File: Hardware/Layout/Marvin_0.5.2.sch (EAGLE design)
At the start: 56 parts, among them IC1 LM321MF, Q1 IRLML5203, Q2 IRLML5203, Q3 IRLML5203, U1 ATMEGA32U4-XUAU, U2 SI2366DS-T1-GE3, U3 SI2366DS-T1-GE3, U4 SI2366DS-T1-GE3, U5 LT1761IS5-3.3TRMPBF, X3 BU-SMA-H, Y1 CSTCE16M0V53-R0 16MHZ

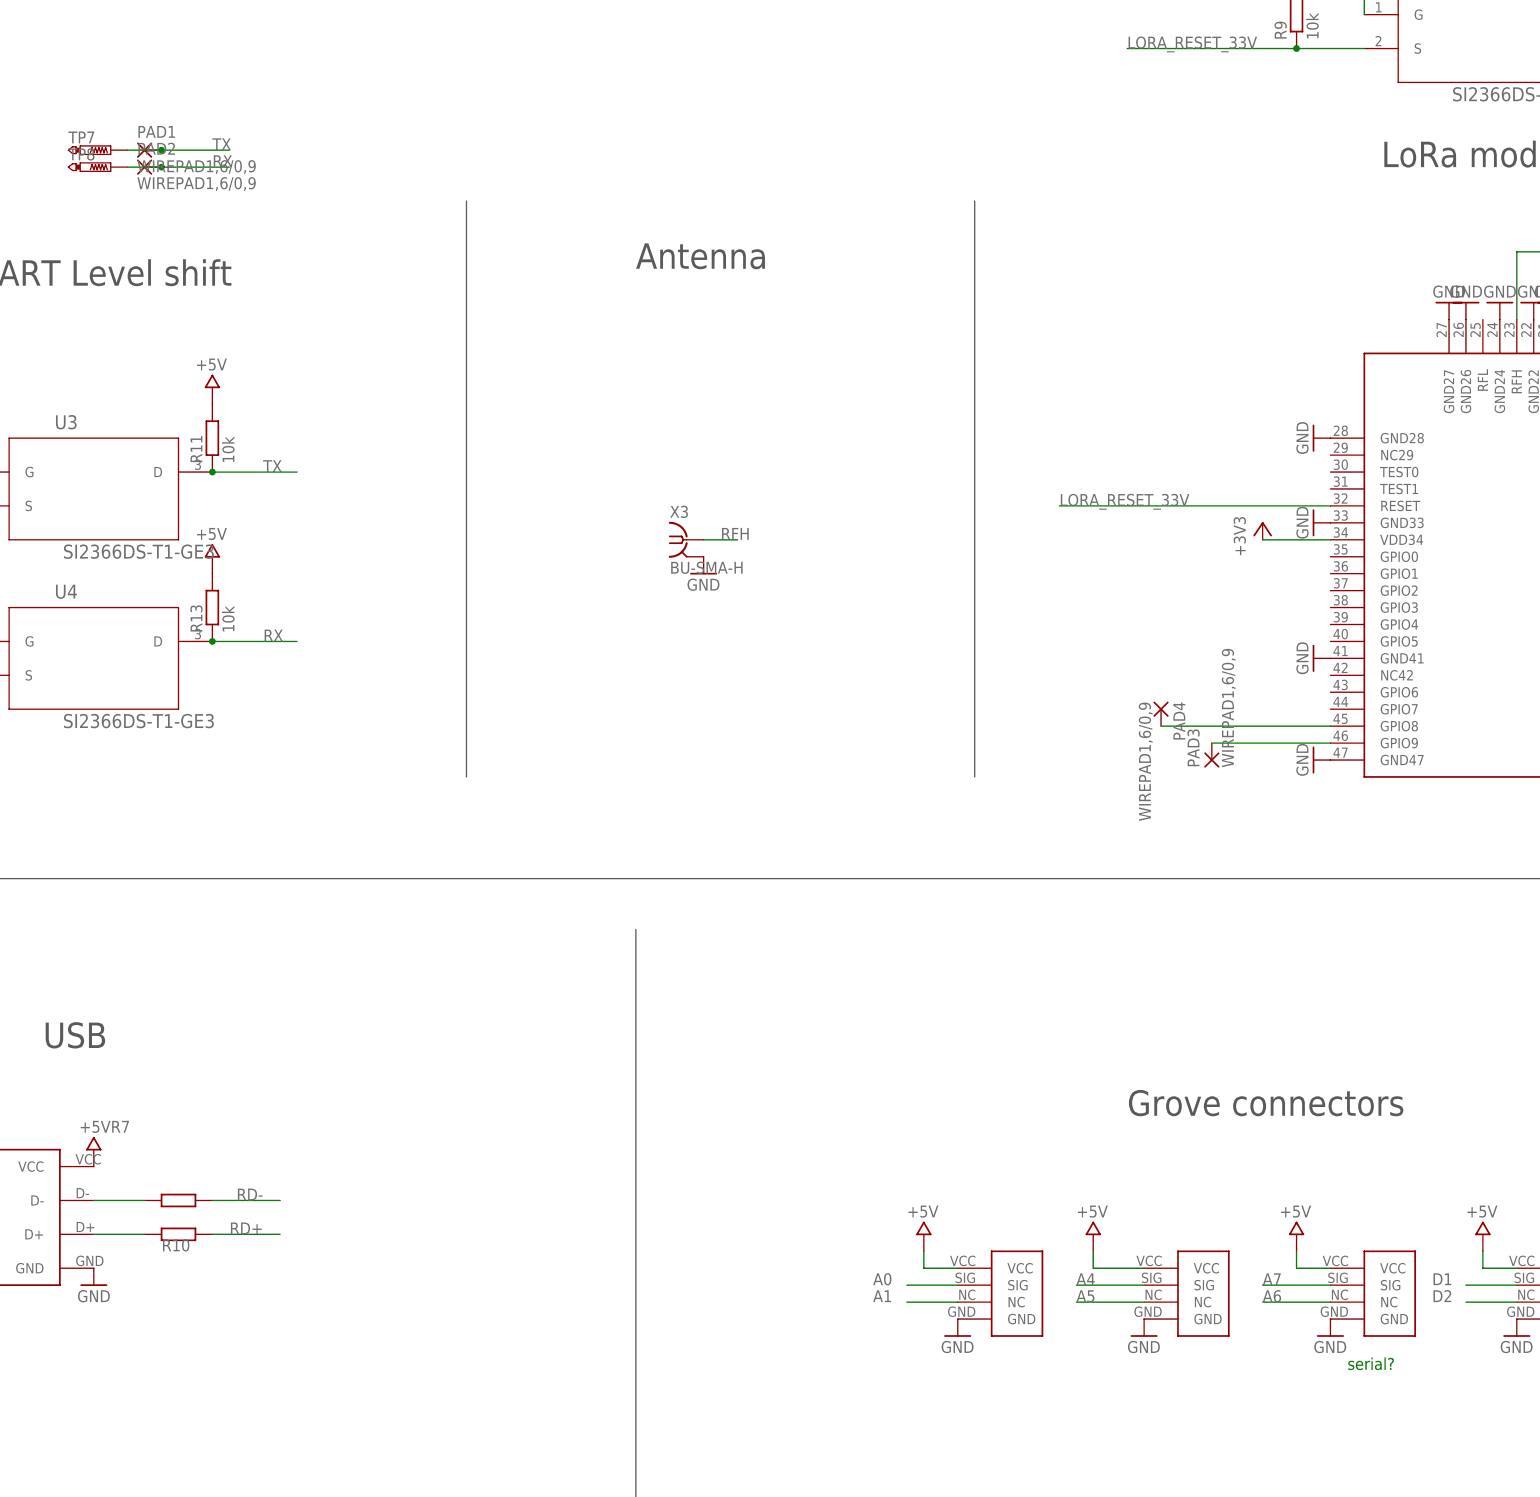
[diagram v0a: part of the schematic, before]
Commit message: brd updates
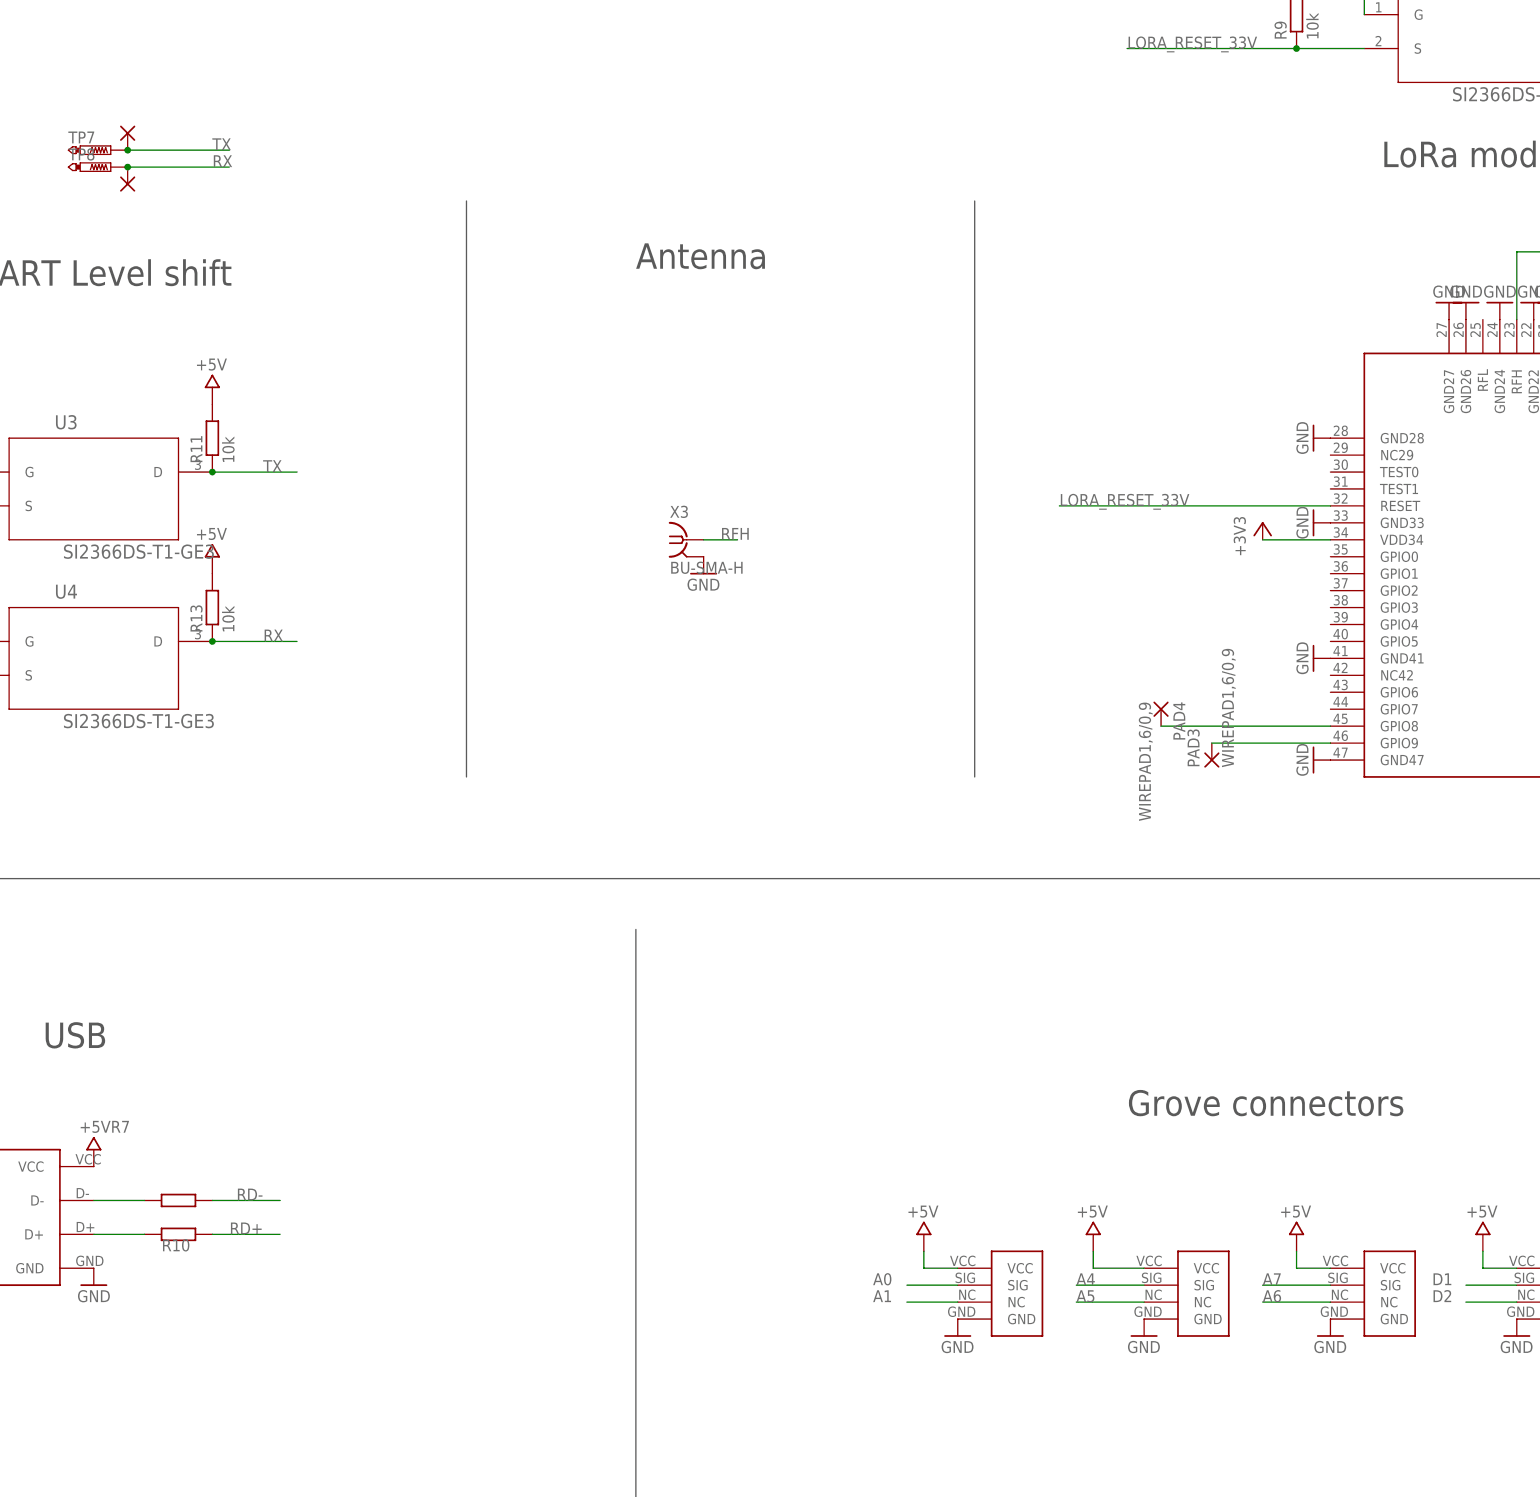
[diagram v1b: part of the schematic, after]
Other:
- note removed: "serial?"
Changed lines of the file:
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@@
 <grid distance="0.1" unitdist="inch" unit="inch" style="lines" multiple="1" display="no" altdistance="0.01" altunitdist="inch" altunit="inch"/>
 <layers>
-<layer number="1" name="Top" color="4" fill="1" visible="yes" active="no"/>
-<layer number="2" name="Route2" color="1" fill="3" visible="yes" active="no"/>
-<layer number="3" name="Route3" color="4" fill="3" visible="yes" active="no"/>
-<layer number="14" name="Route14" color="1" fill="6" visible="yes" active="no"/>
-<layer number="15" name="Route15" color="4" fill="6" visible="yes" active="no"/>
-<layer number="16" name="Bottom" color="1" fill="1" visible="yes" active="no"/>
-<layer number="17" name="Pads" color="2" fill="1" visible="yes" active="no"/>
-<layer number="18" name="Vias" color="2" fill="1" visible="yes" active="no"/>
-<layer number="19" name="Unrouted" color="6" fill="1" visible="yes" active="no"/>
-<layer number="20" name="Dimension" color="15" fill="1" visible="yes" active="no"/>
-<layer number="21" name="tPlace" color="7" fill="1" visible="yes" active="no"/>
-<layer number="22" name="bPlace" color="7" fill="1" visible="yes" active="no"/>
-<layer number="23" name="tOrigins" color="15" fill="1" visible="yes" active="no"/>
-<layer number="24" name="bOrigins" color="15" fill="1" visible="yes" active="no"/>
-<layer number="25" name="tNames" color="7" fill="1" visible="yes" active="no"/>
-<layer number="26" name="bNames" color="7" fill="1" visible="yes" active="no"/>
-<layer number="27" name="tValues" color="7" fill="1" visible="yes" active="no"/>
-<layer number="28" name="bValues" color="7" fill="1" visible="yes" active="no"/>
+<layer number="1" name="Top" color="4" fill="1" visible="no" active="no"/>
+<layer number="2" name="Route2" color="1" fill="3" visible="no" active="no"/>
+<layer number="3" name="Route3" color="4" fill="3" visible="no" active="no"/>
+<layer number="14" name="Route14" color="1" fill="6" visible="no" active="no"/>
+<layer number="15" name="Route15" color="4" fill="6" visible="no" active="no"/>
+<layer number="16" name="Bottom" color="1" fill="1" visible="no" active="no"/>
+<layer number="17" name="Pads" color="2" fill="1" visible="no" active="no"/>
+<layer number="18" name="Vias" color="2" fill="1" visible="no" active="no"/>
+<layer number="19" name="Unrouted" color="6" fill="1" visible="no" active="no"/>
+<layer number="20" name="Dimension" color="15" fill="1" visible="no" active="no"/>
+<layer number="21" name="tPlace" color="7" fill="1" visible="no" active="no"/>
+<layer number="22" name="bPlace" color="7" fill="1" visible="no" active="no"/>
+<layer number="23" name="tOrigins" color="15" fill="1" visible="no" active="no"/>
+<layer number="24" name="bOrigins" color="15" fill="1" visible="no" active="no"/>
+<layer number="25" name="tNames" color="7" fill="1" visible="no" active="no"/>
+<layer number="26" name="bNames" color="7" fill="1" visible="no" active="no"/>
+<layer number="27" name="tValues" color="7" fill="1" visible="no" active="no"/>
+<layer number="28" name="bValues" color="7" fill="1" visible="no" active="no"/>
 <layer number="29" name="tStop" color="7" fill="3" visible="no" active="no"/>
 <layer number="30" name="bStop" color="7" fill="6" visible="no" active="no"/>
@@
 <layer number="35" name="tGlue" color="7" fill="4" visible="no" active="no"/>
 <layer number="36" name="bGlue" color="7" fill="5" visible="no" active="no"/>
-<layer number="37" name="tTest" color="7" fill="1" visible="yes" active="no"/>
-<layer number="38" name="bTest" color="7" fill="1" visible="yes" active="no"/>
+<layer number="37" name="tTest" color="7" fill="1" visible="no" active="no"/>
+<layer number="38" name="bTest" color="7" fill="1" visible="no" active="no"/>
 <layer number="39" name="tKeepout" color="4" fill="11" visible="no" active="no"/>
 <layer number="40" name="bKeepout" color="1" fill="11" visible="no" active="no"/>
@@
 <layer number="44" name="Drills" color="7" fill="1" visible="no" active="no"/>
 <layer number="45" name="Holes" color="7" fill="1" visible="no" active="no"/>
-<layer number="46" name="Milling" color="3" fill="1" visible="yes" active="no"/>
-<layer number="47" name="Measures" color="7" fill="1" visible="yes" active="no"/>
-<layer number="48" name="Document" color="7" fill="1" visible="yes" active="no"/>
-<layer number="49" name="Reference" color="7" fill="1" visible="yes" active="no"/>
-<layer number="50" name="dxf" color="7" fill="1" visible="yes" active="no"/>
-<layer number="51" name="tDocu" color="7" fill="1" visible="yes" active="no"/>
-<layer number="52" name="bDocu" color="7" fill="1" visible="yes" active="no"/>
-<layer number="53" name="tGND_GNDA" color="7" fill="9" visible="yes" active="no"/>
-<layer number="54" name="bGND_GNDA" color="1" fill="9" visible="yes" active="no"/>
-<layer number="56" name="wert" color="7" fill="1" visible="yes" active="no"/>
-<layer number="57" name="tCAD" color="7" fill="1" visible="yes" active="no"/>
-<layer number="59" name="tCarbon" color="7" fill="1" visible="yes" active="no"/>
-<layer number="60" name="bCarbon" color="7" fill="1" visible="yes" active="no"/>
+<layer number="46" name="Milling" color="3" fill="1" visible="no" active="no"/>
+<layer number="47" name="Measures" color="7" fill="1" visible="no" active="no"/>
+<layer number="48" name="Document" color="7" fill="1" visible="no" active="no"/>
+<layer number="49" name="Reference" color="7" fill="1" visible="no" active="no"/>
+<layer number="50" name="dxf" color="7" fill="1" visible="no" active="no"/>
+<layer number="51" name="tDocu" color="7" fill="1" visible="no" active="no"/>
+<layer number="52" name="bDocu" color="7" fill="1" visible="no" active="no"/>
+<layer number="53" name="tGND_GNDA" color="7" fill="9" visible="no" active="no"/>
+<layer number="54" name="bGND_GNDA" color="1" fill="9" visible="no" active="no"/>
+<layer number="56" name="wert" color="7" fill="1" visible="no" active="no"/>
+<layer number="57" name="tCAD" color="7" fill="1" visible="no" active="no"/>
+<layer number="59" name="tCarbon" color="7" fill="1" visible="no" active="no"/>
+<layer number="60" name="bCarbon" color="7" fill="1" visible="no" active="no"/>
 <layer number="90" name="Modules" color="5" fill="1" visible="yes" active="yes"/>
 <layer number="91" name="Nets" color="2" fill="1" visible="yes" active="yes"/>
@@
 <text x="106.68" y="78.74" size="3.81" layer="97">ATMEGA32u4</text>
 <text x="22.86" y="12.7" size="3.81" layer="97">ISP header</text>
-<text x="246.38" y="121.92" size="1.778" layer="91">serial?</text>
 </plain>
 <instances>
@@
 <instance part="R1" gate="G$1" x="254" y="66.04" rot="R90"/>
 <instance part="U$22" gate="G$1" x="254" y="73.66"/>
-<instance part="PAD1" gate="G$1" x="66.04" y="304.8"/>
-<instance part="PAD2" gate="G$1" x="66.04" y="302.26"/>
+<instance part="PAD1" gate="G$1" x="63.5" y="307.34" smashed="yes" rot="R270"/>
+<instance part="PAD2" gate="G$1" x="63.5" y="299.72" smashed="yes" rot="R90"/>
 <instance part="TP7" gate="G$1" x="60.96" y="304.8" rot="R270"/>
 <instance part="TP8" gate="G$1" x="60.96" y="302.26" rot="R270"/>
@@
 <segment>
 <label x="76.2" y="302.26" size="1.778" layer="95"/>
-<wire x1="78.74" y1="302.26" x2="68.58" y2="302.26" width="0.1524" layer="91"/>
+<wire x1="78.74" y1="302.26" x2="63.5" y2="302.26" width="0.1524" layer="91"/>
 <pinref part="PAD2" gate="G$1" pin="P"/>
-<wire x1="68.58" y1="302.26" x2="63.5" y2="302.26" width="0.1524" layer="91"/>
-<junction x="68.58" y="302.26"/>
+<junction x="63.5" y="302.26"/>
 <pinref part="TP8" gate="G$1" pin="TP"/>
 </segment>
@@
 <segment>
 <label x="76.2" y="304.8" size="1.778" layer="95"/>
-<wire x1="78.74" y1="304.8" x2="68.58" y2="304.8" width="0.1524" layer="91"/>
+<wire x1="78.74" y1="304.8" x2="63.5" y2="304.8" width="0.1524" layer="91"/>
 <pinref part="PAD1" gate="G$1" pin="P"/>
-<wire x1="68.58" y1="304.8" x2="63.5" y2="304.8" width="0.1524" layer="91"/>
-<junction x="68.58" y="304.8"/>
+<junction x="63.5" y="304.8"/>
 <pinref part="TP7" gate="G$1" pin="TP"/>
 </segment>
